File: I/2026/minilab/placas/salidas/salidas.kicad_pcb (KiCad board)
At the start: 2 copper layers, 36.5 x 39 mm, 26 parts, among them SW1 SW_DPST_x2, SW2 SW_DPST_x2, SW3 SW_DPST_x2, SW4 SW_DPST_x2, SW5 SW_DPST_x2, SW6 SW_DPST_x2

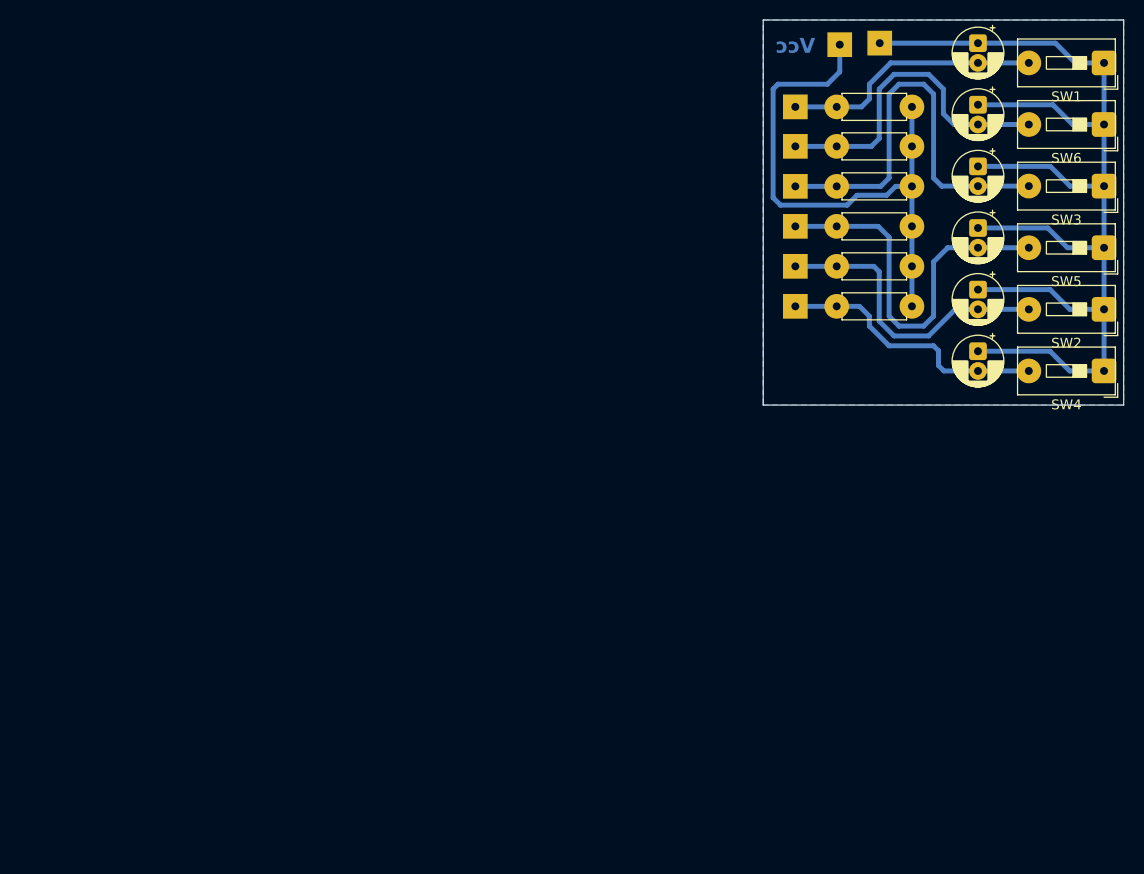
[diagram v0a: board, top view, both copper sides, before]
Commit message: check entradas
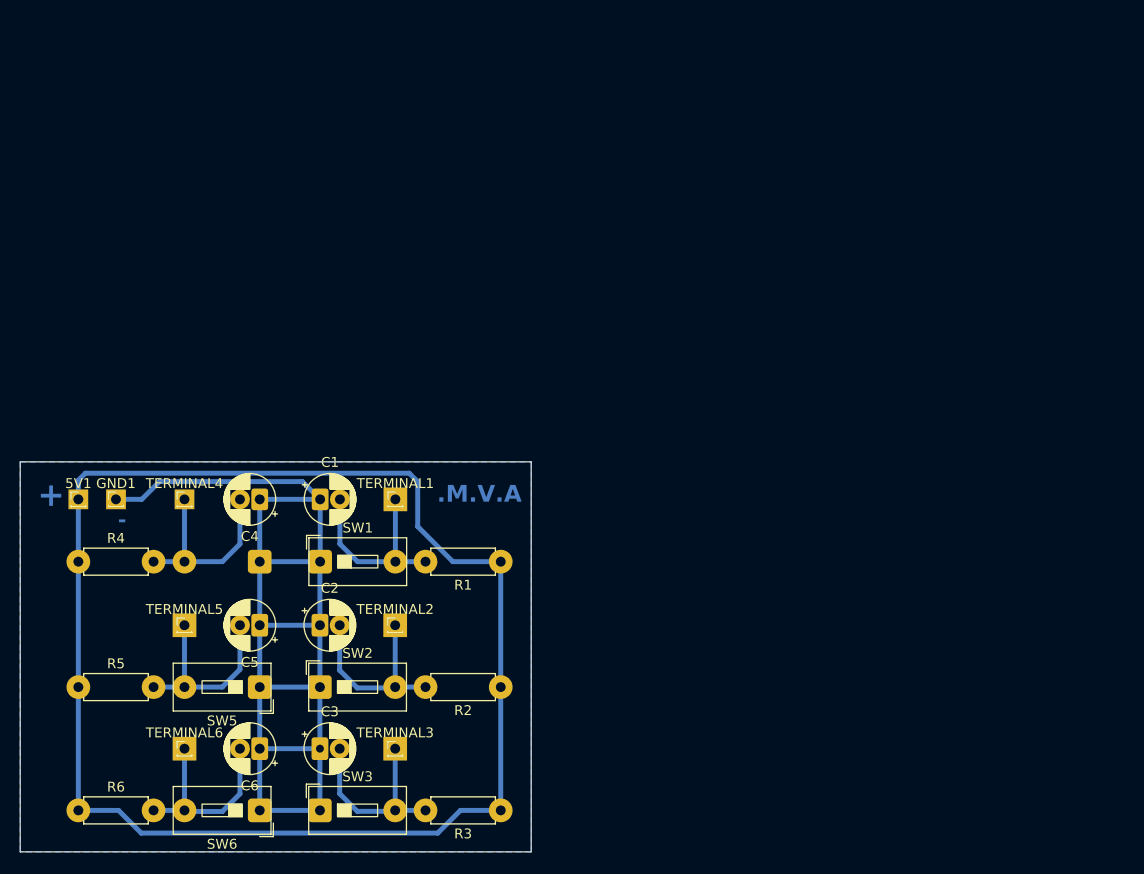
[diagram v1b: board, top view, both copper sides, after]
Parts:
- 5V1, GND1, TERMINAL1, TERMINAL2, TERMINAL3, TERMINAL4, TERMINAL5, TERMINAL6: footprint Library:PinHeader_1x01_P1.00mm_VerticalBIG -> Connector_PinHeader_1.00mm:PinHeader_1x01_P1.00mm_Vertical
- C1, C2, C3, C4, C5, C6: footprint Library:CP_Radial_D5.0mm_P2.00mmBIG -> Capacitor_THT:CP_Radial_D5.0mm_P2.00mm
- R1, R2, R3, R4, R5, R6: footprint Library:R_Axial_DIN0207_L6.3mm_D2.5mm_P7.62mm_HorizontalBIG -> Resistor_THT:R_Axial_DIN0207_L6.3mm_D2.5mm_P7.62mm_Horizontal
- SW1, SW2, SW3, SW5, SW6: footprint Library:SW_DIP_SPSTx01_Slide_9.78x4.72mm_W7.62mm_P2.54mmBIG -> Button_Switch_THT:SW_DIP_SPSTx01_Slide_9.78x4.72mm_W7.62mm_P2.54mm
- SW4: footprint Library:SW_DIP_SPSTx01_Slide_9.78x4.72mm_W7.62mm_P2.54mmBIG -> Button_Switch_THT:SW_DIP_SPSTx01_Slide_9.78x4.72mm_W7.62mm_P2.54mm; moved to B.Cu
- moved SW6 110.2 mm to (88.3, 94.5)
- moved R6 107.9 mm to (69.9, 94.5), turned to 0 degrees
- moved SW3 101.5 mm to (94.4, 94.5), turned to 0 degrees
- moved R5 98.5 mm to (69.9, 82.1), turned to 0 degrees
- moved C6 97.7 mm to (88.3, 88.3), turned to 180 degrees
- moved SW5 96.4 mm to (88.3, 82.1)
- moved SW1 94.1 mm to (94.4, 69.4), turned to 0 degrees
- moved R4 91.0 mm to (69.9, 69.4), turned to 0 degrees
- moved GND1 90.1 mm to (73.7, 63.0), turned to 0 degrees
- moved 5V1 89.8 mm to (69.9, 63.0), turned to 0 degrees
- moved SW2 88.1 mm to (94.4, 82.1), turned to 0 degrees
- moved SW4 87.7 mm to (88.3, 69.4)
- moved TERMINAL6 86.9 mm to (80.6, 88.3)
- moved C5 86.3 mm to (88.3, 75.8), turned to 180 degrees
- moved C3 81.3 mm to (94.4, 88.3), turned to 0 degrees
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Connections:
- C2 pad 2: Net-(SW4A-B) -> Net-(SW2A-B)
- C3 pad 2: Net-(SW2A-B) -> Net-(SW3A-B)
- C4 pad 2: Net-(SW5A-B) -> Net-(SW4A-B)
- C5 pad 2: Net-(SW3A-B) -> Net-(SW5A-B)
- R2 pad 2: Net-(SW4A-B) -> Net-(SW2A-B)
- R3 pad 2: Net-(SW2A-B) -> Net-(SW3A-B)
- R4 pad 2: Net-(SW5A-B) -> Net-(SW4A-B)
- R5 pad 2: Net-(SW3A-B) -> Net-(SW5A-B)
- TERMINAL2 pad 1: Net-(SW4A-B) -> Net-(SW2A-B)
- TERMINAL3 pad 1: Net-(SW2A-B) -> Net-(SW3A-B)
- TERMINAL4 pad 1: Net-(SW5A-B) -> Net-(SW4A-B)
- TERMINAL5 pad 1: Net-(SW3A-B) -> Net-(SW5A-B)
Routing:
- net Net-(5V1-Pin_1): track 56.6 -> 152.5 mm
- net Net-(SW3A-B): track 42.4 -> 20.2 mm
- net Net-(SW5A-B): track 39.2 -> 20.3 mm
- net Net-(SW6A-B): track 33.5 -> 20.3 mm
- net Net-(SW2A-B): track 30.7 -> 20.2 mm
- net Net-(SW4A-B): track 27.8 -> 20.3 mm
- net Net-(SW1A-B): track 26.7 -> 20.2 mm
- net Net-(GND1-Pin_1): track 122.7 -> 121.9 mm
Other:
- board size 36.5 x 39 mm -> 51.8 x 39.5 mm
- board text added: "+"
- board text added: "-"
- board text added: "A.V.M."
- board text removed: "Vcc"
